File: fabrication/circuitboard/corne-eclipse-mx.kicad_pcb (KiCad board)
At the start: 2 copper layers, 275.5 x 105.6 mm, 182 parts, among them J2 OLED, J4 OLED, Q1 AO3401A, Q2 AO3401A, SW1 SW_MX_HS, SW10 SW_MX_HS, SW11 SW_MX_HS, SW12 SW_MX_HS, SW13 SW_MX_HS, SW14 SW_MX_HS, SW15 SW_MX_HS, SW16 SW_MX_HS, SW17 SW_MX_HS, SW18 SW_MX_HS, SW2 SW_MX_HS, SW20 SW_MX_HS, SW21 SW_MX_HS, SW22 SW_MX_HS, SW23 SW_MX_HS, SW24 SW_MX_HS, SW25 SW_MX_HS, SW26 SW_MX_HS, SW27 SW_MX_HS, SW28 SW_MX_HS, SW29 SW_MX_HS, SW3 SW_MX_HS, SW30 SW_MX_HS, SW31 SW_MX_HS, SW32 SW_MX_HS, SW33 SW_MX_HS, SW34 SW_MX_HS, SW35 SW_MX_HS, SW36 SW_MX_HS, SW37 SW_MX_HS, SW38 SW_MX_HS, SW39 SW_MX_HS, SW4 SW_MX_HS, SW40 SW_MX_HS, SW42 SW_MX_HS, SW43 SW_MX_HS, SW44 SW_MX_HS, SW5 SW_MX_HS, SW6 SW_MX_HS, SW7 SW_MX_HS, SW8 SW_MX_HS, SW9 SW_MX_HS, U1 nice!nano, U2 nice!nano

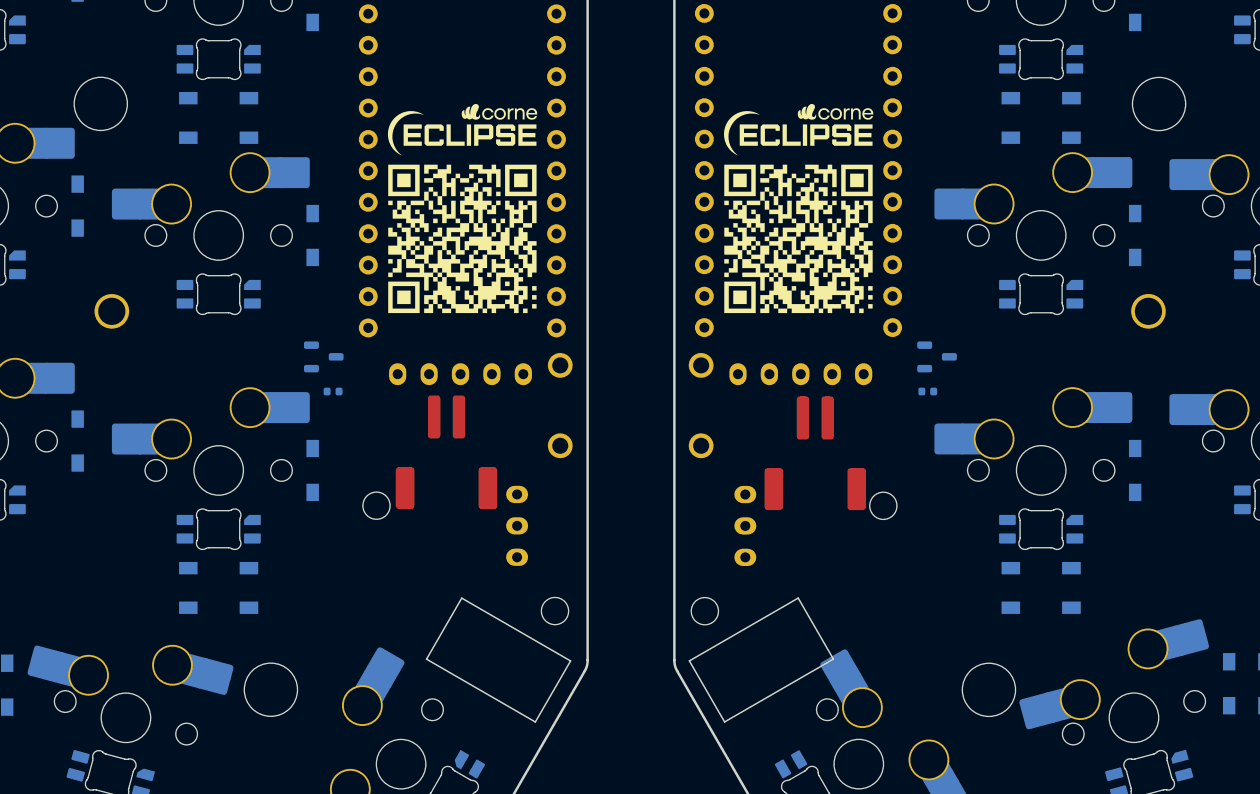
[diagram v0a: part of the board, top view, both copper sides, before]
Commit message: wip
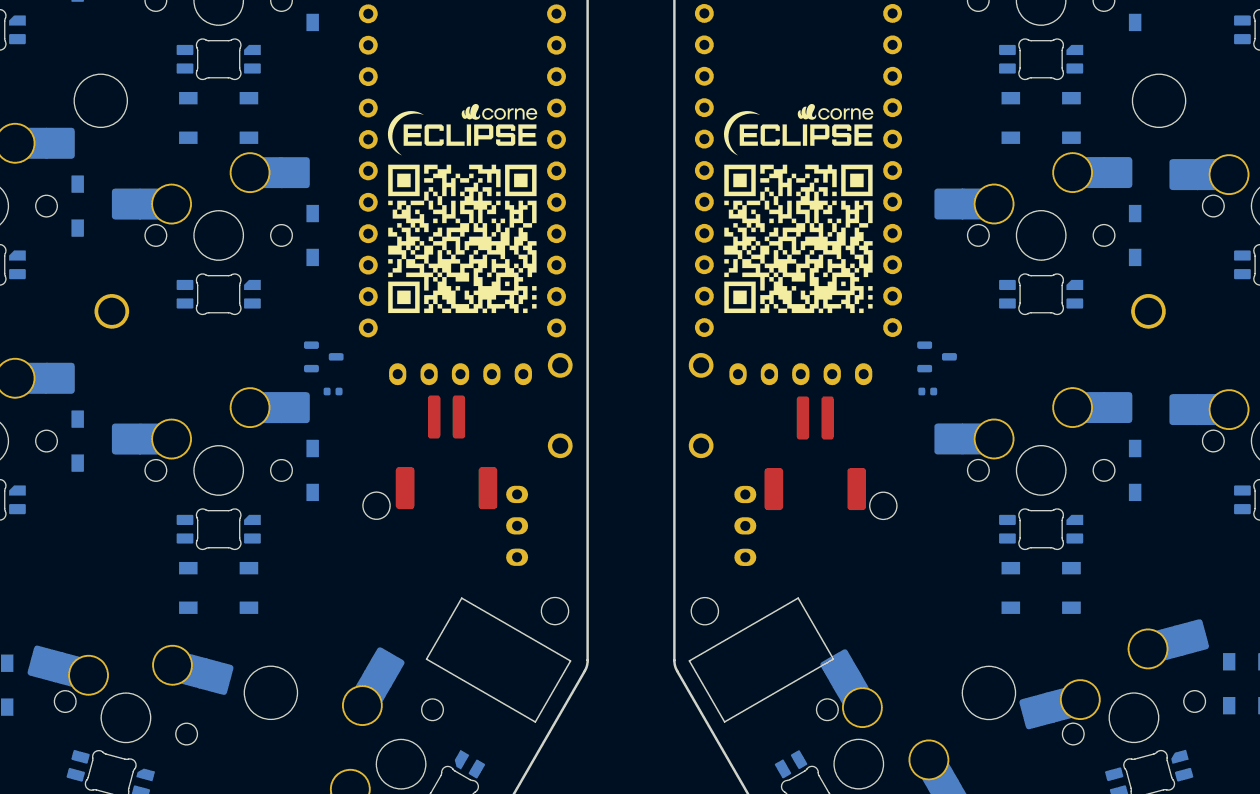
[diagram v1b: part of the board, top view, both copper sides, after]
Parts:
- moved MH3 0.25 mm to (119.3, 88.4)
- moved MH6 0.25 mm to (177.4, 88.4)
